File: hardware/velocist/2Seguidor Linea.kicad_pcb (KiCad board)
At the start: 2 copper layers, 140 x 158.4 mm, 19 parts, among them J1 XT30, J2 Cable_PAD, J3 Cable_PAD, J4 QTR8a, SW1 SW_Push, SW3 SW_SPDT, U1 TB6612FNG, U2 Mini360, U3 ESP32_DEVKITC

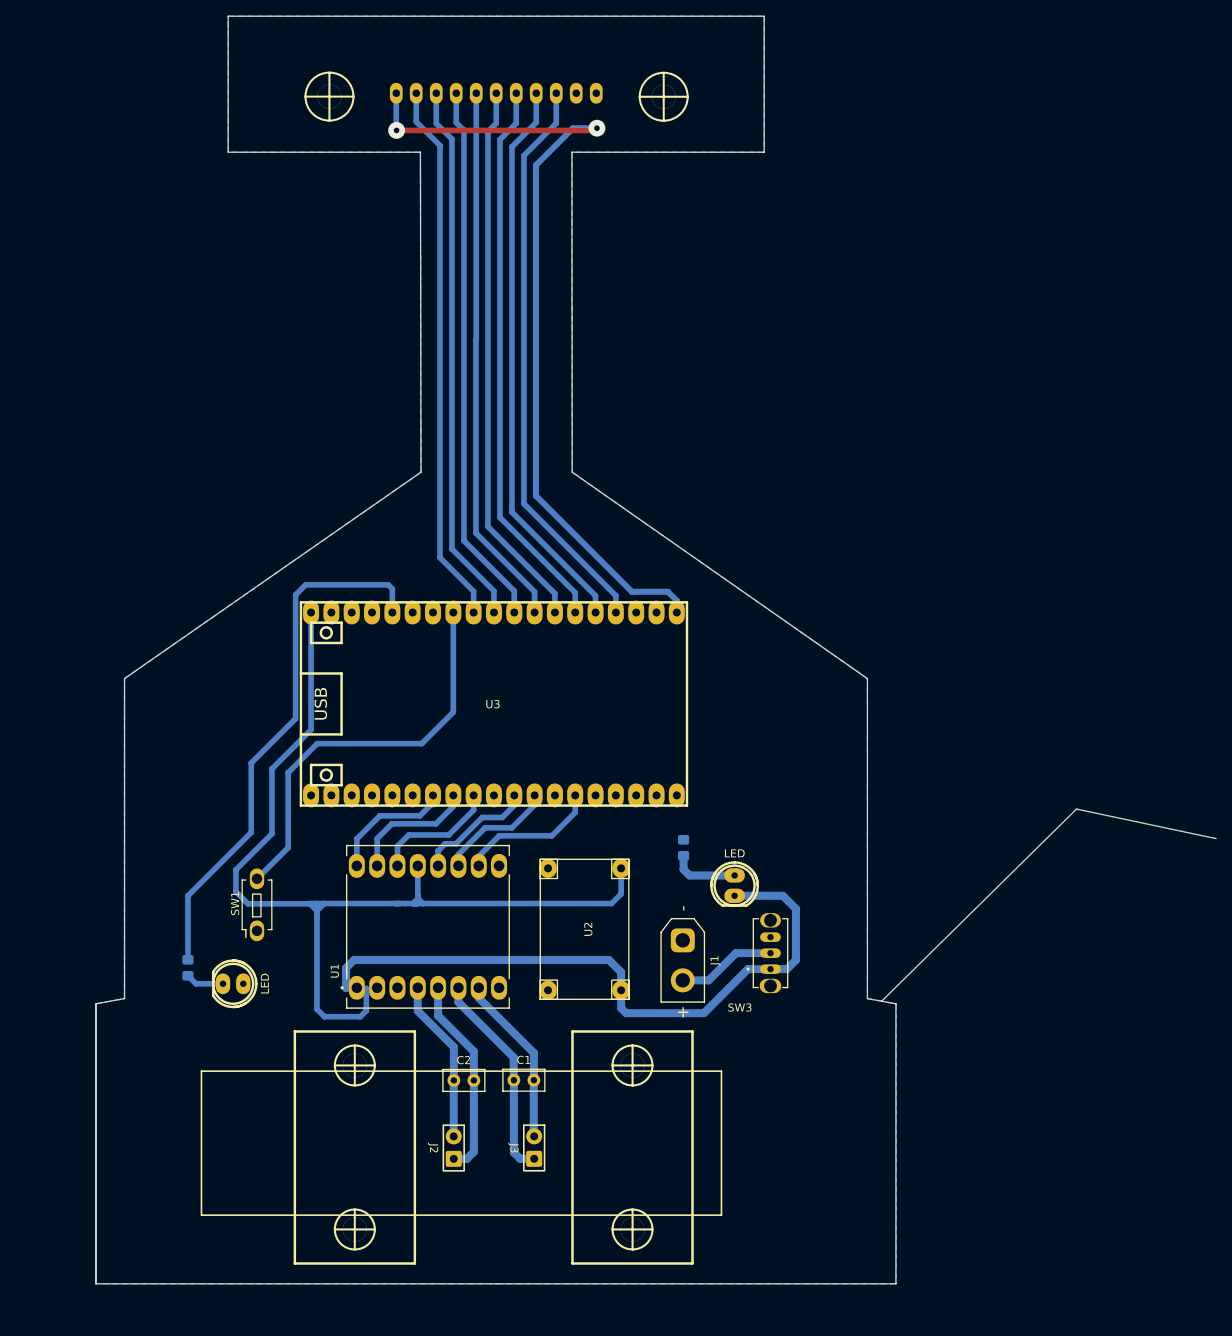
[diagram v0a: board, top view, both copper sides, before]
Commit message: act placa
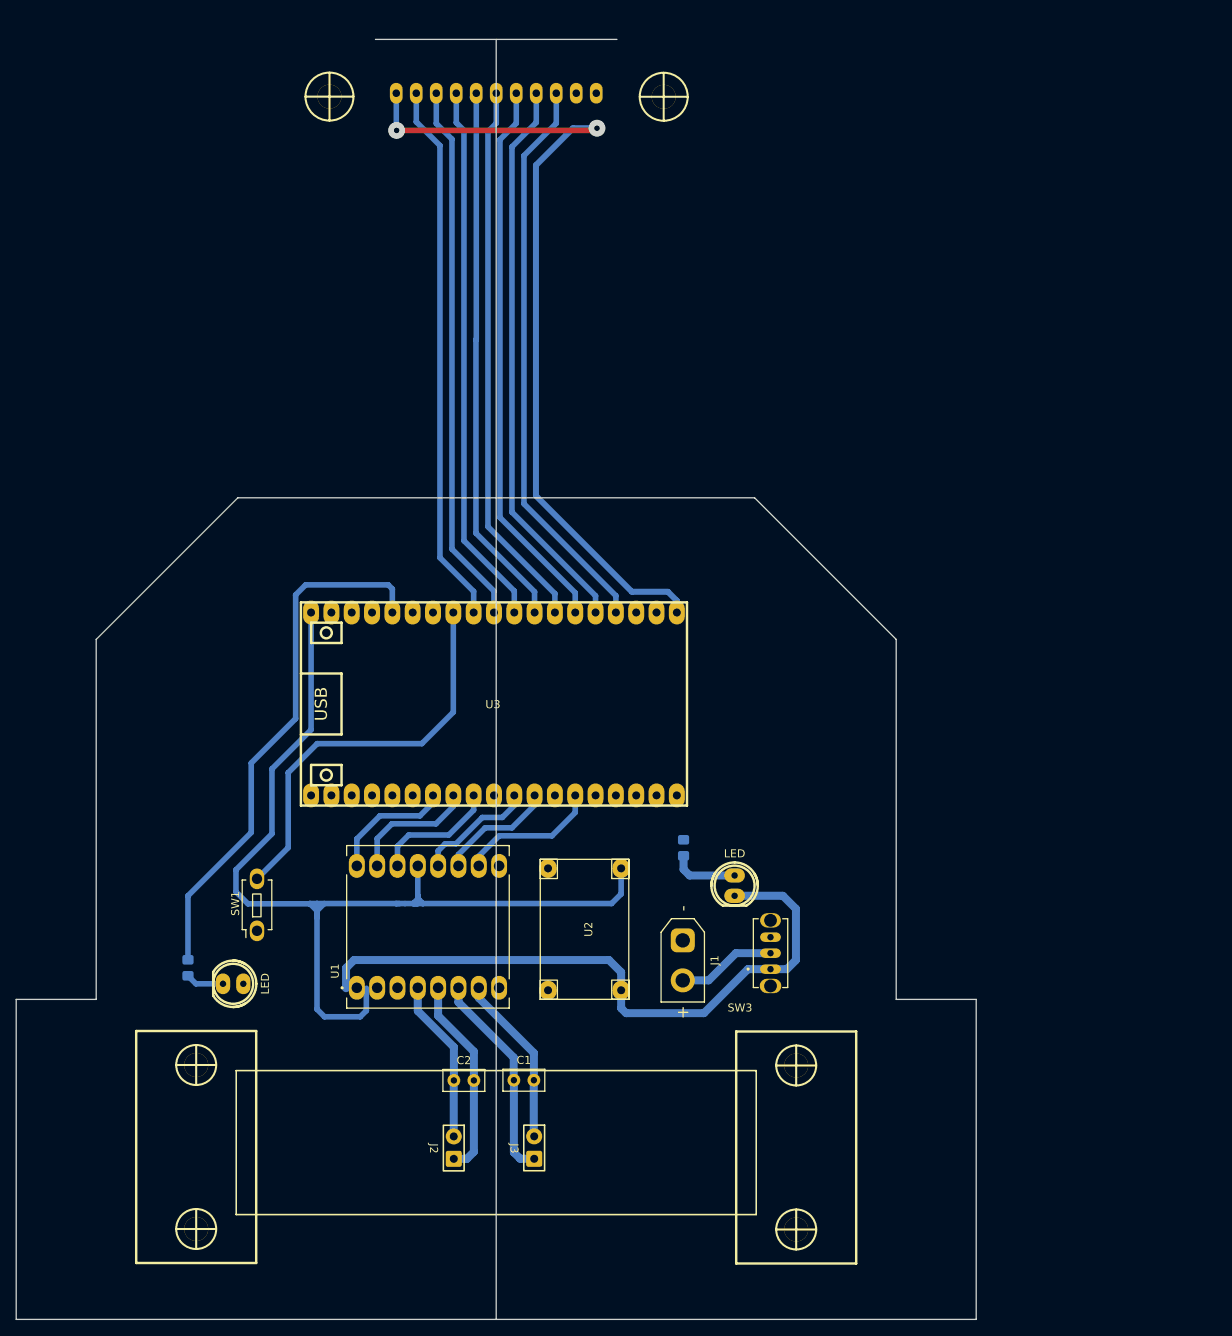
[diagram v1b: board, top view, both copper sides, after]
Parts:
- moved Pololu_Micro_Gear_Motor 20.5 mm to (136.0, 167.4)
- moved Pololu_Micro_Gear_Motor 19.8 mm to (61.0, 167.3)
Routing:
- removed copper zone on B.Cu, net GND
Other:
- board size 140 x 158.4 mm -> 120 x 160 mm
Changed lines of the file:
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@@
 	(footprint "Bracket:Pololu_Micro_Bracket_Wheel_42mm"
 		(layer "F.Cu")
-		(at 115.54 167.41 -90)
+		(at 136 167.41 -90)
 		(descr "Pololu Micro Gear Motor W/Mount")
 		(property "Reference" "Pololu_Micro_Gear_Motor"
@@
 	(footprint "Bracket:Pololu_Micro_Bracket_Wheel_42mm"
 		(layer "F.Cu")
-		(at 80.83 167.41 90)
+		(at 61 167.35 90)
 		(descr "Pololu Micro Gear Motor W/Mount")
 		(property "Reference" "Pololu_Micro_Gear_Motor"
@@
 	)
 	(gr_rect
-		(start 61.66 157.87)
-		(end 126.66 175.87)
+		(start 66 157.8)
+		(end 131 175.8)
 		(stroke
 			(width 0.2)
@@
 	)
 	(gr_line
-		(start 132 43)
-		(end 132 26)
+		(start 48.5 148.9)
+		(end 48.5 103.9)
 		(stroke
 			(width 0.05)
@@
 	)
 	(gr_line
-		(start 98.5 26)
-		(end 65 26)
+		(start 158.5 188.9)
+		(end 158.5 148.9)
 		(stroke
 			(width 0.05)
@@
 	)
 	(gr_line
-		(start 107.97 43)
-		(end 132 43)
+		(start 38.5 188.9)
+		(end 38.5 148.9)
 		(stroke
 			(width 0.05)
@@
 	)
 	(gr_line
-		(start 52.04 108.8)
-		(end 52.04 148.8)
+		(start 148.5 148.9)
+		(end 148.5 103.9)
 		(stroke
 			(width 0.05)
@@
 	)
 	(gr_line
-		(start 148.47 184.45)
-		(end 148.47 149.45)
+		(start 38.5 148.9)
+		(end 48.5 148.9)
 		(stroke
 			(width 0.05)
@@
 	)
 	(gr_line
-		(start 52.04 148.8)
-		(end 48.47 149.45)
+		(start 158.5 148.9)
+		(end 148.5 148.9)
 		(stroke
 			(width 0.05)
@@
 	)
 	(gr_line
-		(start 144.9 148.8)
-		(end 148.47 149.45)
+		(start 38.5 188.9)
+		(end 158.5 188.9)
 		(stroke
 			(width 0.05)
@@
 	)
 	(gr_line
-		(start 144.9 108.8)
-		(end 144.9 148.8)
+		(start 83.4 28.9)
+		(end 113.6 28.9)
 		(stroke
 			(width 0.05)
@@
 	)
 	(gr_line
-		(start 188.48 128.8)
-		(end 171.04 125.11)
+		(start 148.5 103.9)
+		(end 130.8 86.2)
 		(stroke
 			(width 0.05)
@@
 	)
 	(gr_line
-		(start 107.97 43)
-		(end 108 83)
+		(start 98.5 28.9)
+		(end 98.5 188.9)
 		(stroke
 			(width 0.05)
@@
 	)
 	(gr_line
-		(start 89.03 43)
-		(end 65 43)
+		(start 66.2 86.2)
+		(end 130.8 86.2)
 		(stroke
 			(width 0.05)
@@
 	)
 	(gr_line
-		(start 108 83)
-		(end 144.9 108.8)
-		(stroke
-			(width 0.05)
-			(type default)
-		)
-		(layer "Edge.Cuts")
-	)
-	(gr_line
-		(start 48.47 149.45)
-		(end 48.47 184.45)
-		(stroke
-			(width 0.05)
-			(type default)
-		)
-		(layer "Edge.Cuts")
-	)
-	(gr_line
-		(start 98.47 184.45)
-		(end 48.47 184.45)
-		(stroke
-			(width 0.05)
-			(type default)
-		)
-		(layer "Edge.Cuts")
-	)
-	(gr_line
-		(start 98.47 184.45)
-		(end 148.47 184.45)
-		(stroke
-			(width 0.05)
-			(type default)
-		)
-		(layer "Edge.Cuts")
-	)
-	(gr_line
-		(start 171.04 125.11)
-		(end 146.685 149.125)
-		(stroke
-			(width 0.05)
-			(type default)
-		)
-		(layer "Edge.Cuts")
-	)
-	(gr_line
-		(start 48.47 184.45)
-		(end 48.47 149.45)
-		(stroke
-			(width 0.05)
-			(type default)
-		)
-		(layer "Edge.Cuts")
-	)
-	(gr_line
-		(start 98.5 26)
-		(end 132 26)
-		(stroke
-			(width 0.05)
-			(type default)
-		)
-		(layer "Edge.Cuts")
-	)
-	(gr_line
-		(start 89.03 43)
-		(end 89.1 83)
-		(stroke
-			(width 0.05)
-			(type default)
-		)
-		(layer "Edge.Cuts")
-	)
-	(gr_line
-		(start 65 43)
-		(end 65 26)
-		(stroke
-			(width 0.05)
-			(type default)
-		)
-		(layer "Edge.Cuts")
-	)
-	(gr_line
-		(start 89.1 83)
-		(end 52.04 108.8)
+		(start 48.5 103.9)
+		(end 66.2 86.2)
 		(stroke
 			(width 0.05)
@@
 		(net 42)
 	)
-	(zone
-		(net 6)
-		(net_name "GND")
-		(layer "B.Cu")
-		(hatch edge 0.5)
-		(connect_pads
-			(clearance 0.5)
-		)
-		(min_thickness 0.25)
-		(filled_areas_thickness no)
-		(fill yes
-			(thermal_gap 0.5)
-			(thermal_bridge_width 0.5)
-		)
-		(polygon
-			(pts
-				(xy 132 26) (xy 132 43) (xy 107.97 43) (xy 108 83) (xy 144.9 108.8) (xy 144.9 148.8) (xy 148.47 149.45)
-				(xy 148.47 184.45) (xy 48.47 184.45) (xy 48.47 149.45) (xy 52.04 148.8) (xy 52.04 108.8) (xy 89.1 83)
-				(xy 89.03 43) (xy 65 43) (xy 65 26)
-			)
-		)
-	)
 	(embedded_fonts no)
